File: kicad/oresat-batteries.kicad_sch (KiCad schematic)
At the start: 11 parts, among them J1 J-SAMTEC-TFM-120-X1-XXX-D-RA, SW1 D2F-L3-D (LEFT), SW2 D2F-L3-D (RIGHT), SW3 D2F-L3-D (LEFT), SW4 D2F-L3-D (RIGHT)

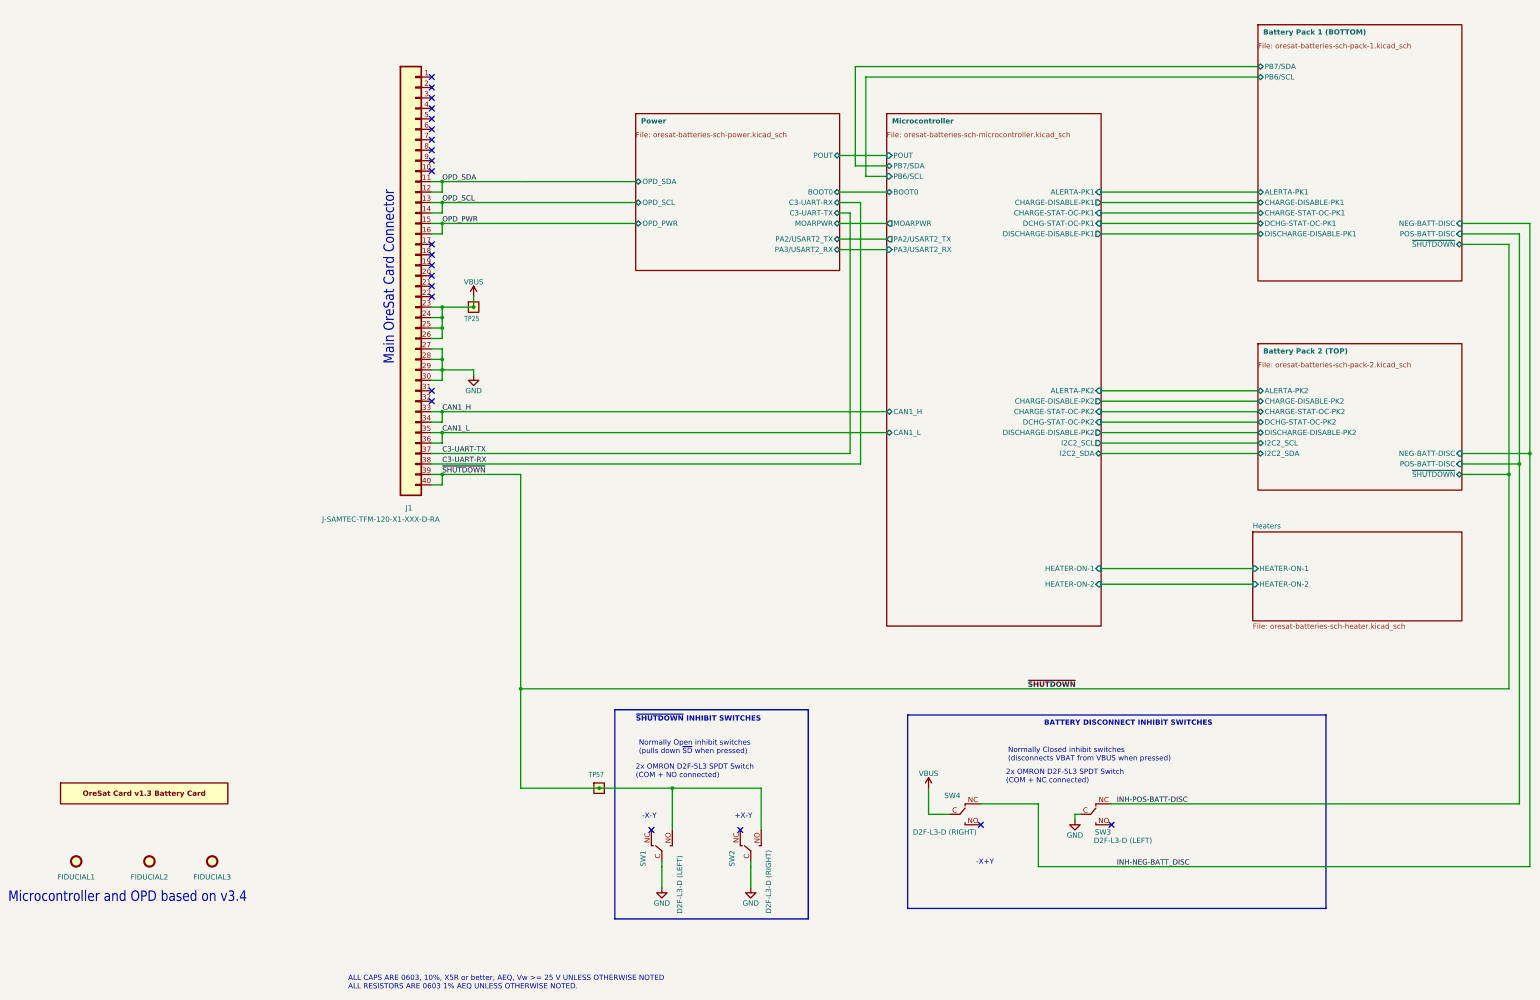
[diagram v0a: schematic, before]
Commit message: Updated data, spiffed up the root page, renamed some STM specific OPD signals, synced SCH and BRD, fixed a bunch of DRC errors, NOW ready for MCXN import that will screw everything up.
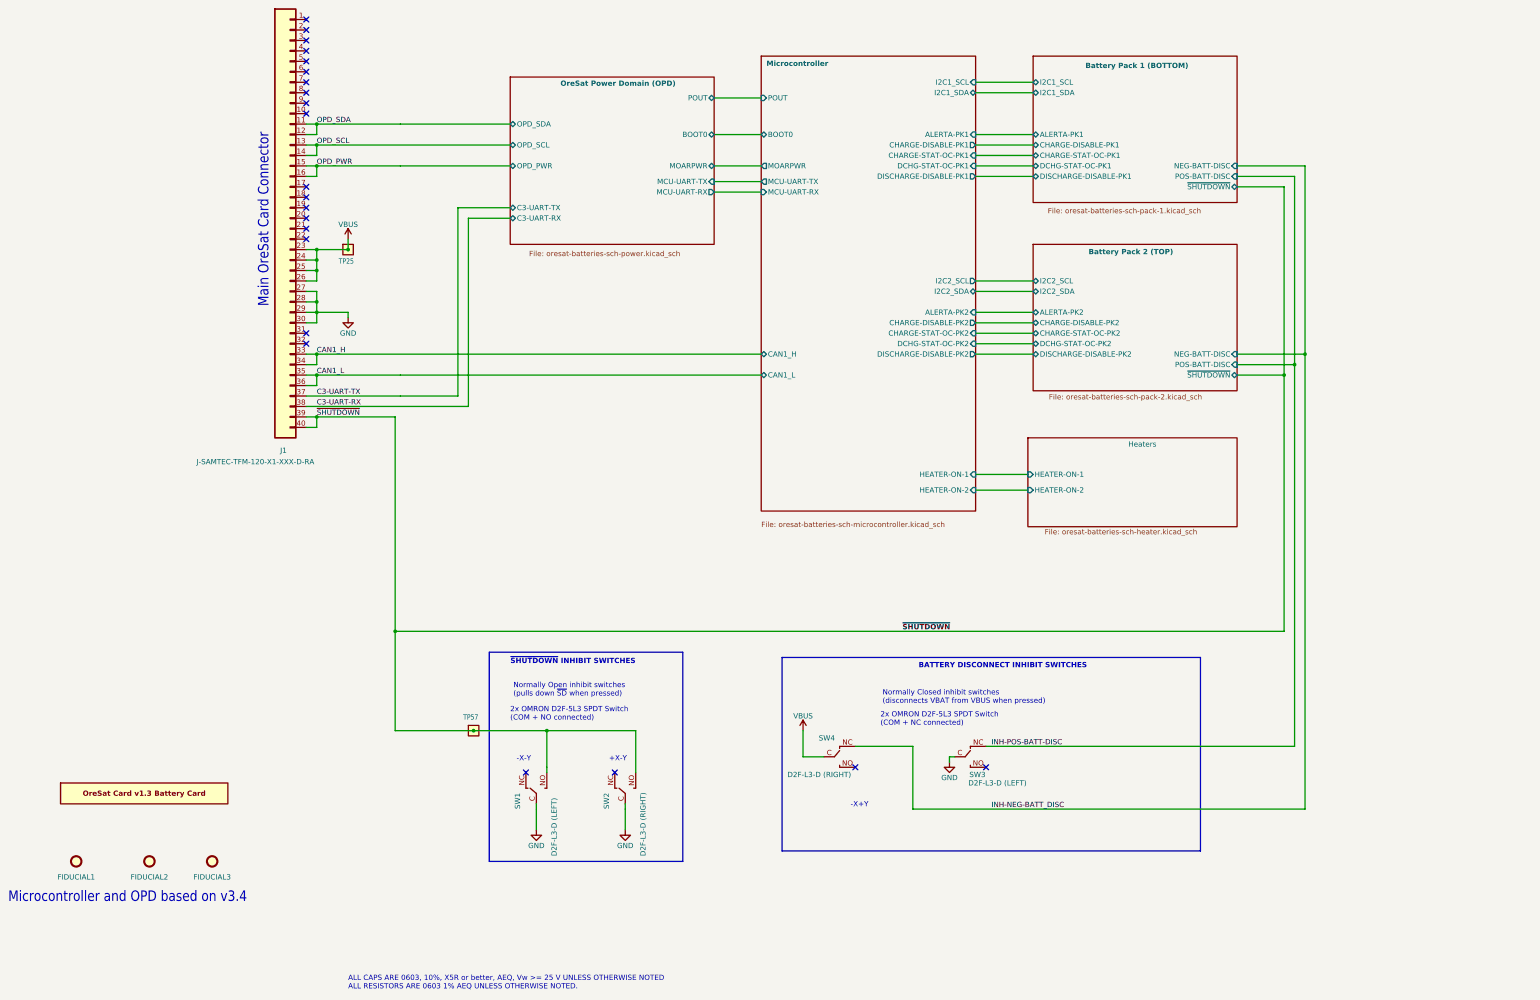
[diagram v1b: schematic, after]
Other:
- sheet Power renamed OreSat Power Domain (OPD)
- sheet Battery Pack 1 (BOTTOM) ports: added I2C1_SCL, I2C1_SDA; removed PB6/SCL, PB7/SDA
- sheet Microcontroller ports: added I2C1_SCL, I2C1_SDA, MCU-UART-RX, MCU-UART-TX; removed PA2/USART2_TX, PA3/USART2_RX, PB6/SCL, PB7/SDA
- sheet OreSat Power Domain (OPD) ports: added MCU-UART-RX, MCU-UART-TX; removed PA2/USART2_TX, PA3/USART2_RX
- moved on the sheet: J1, SW1, SW2, SW3, SW4, TP25, TP57
